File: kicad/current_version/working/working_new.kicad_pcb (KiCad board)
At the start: 2 copper layers, 34 parts, among them J1 bbat328, J2 hi12x3p, J3 scumnsmo, U1 itq32at328, U2 pms22311171d5v, U3 isp16ch340g, X1 xcr3213mhz16, X2 xcr3213mhz12

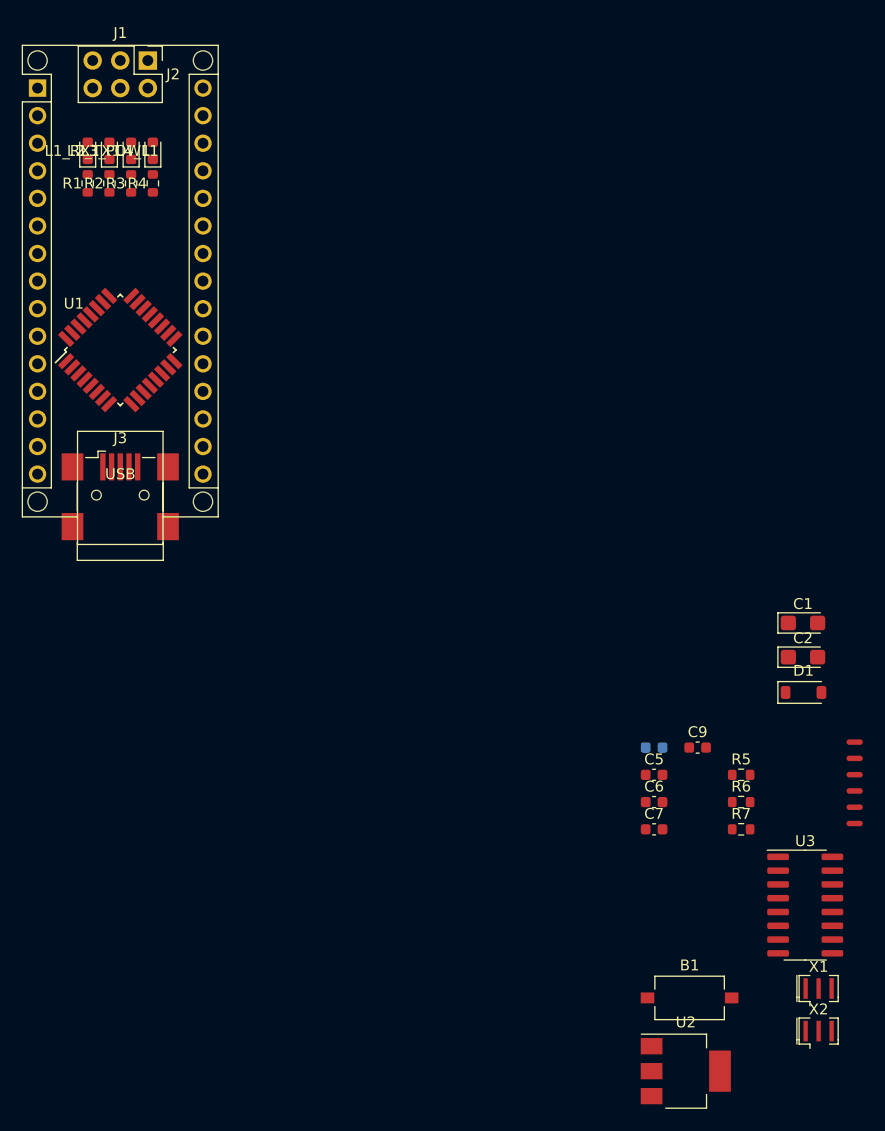
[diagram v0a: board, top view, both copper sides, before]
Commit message: workings
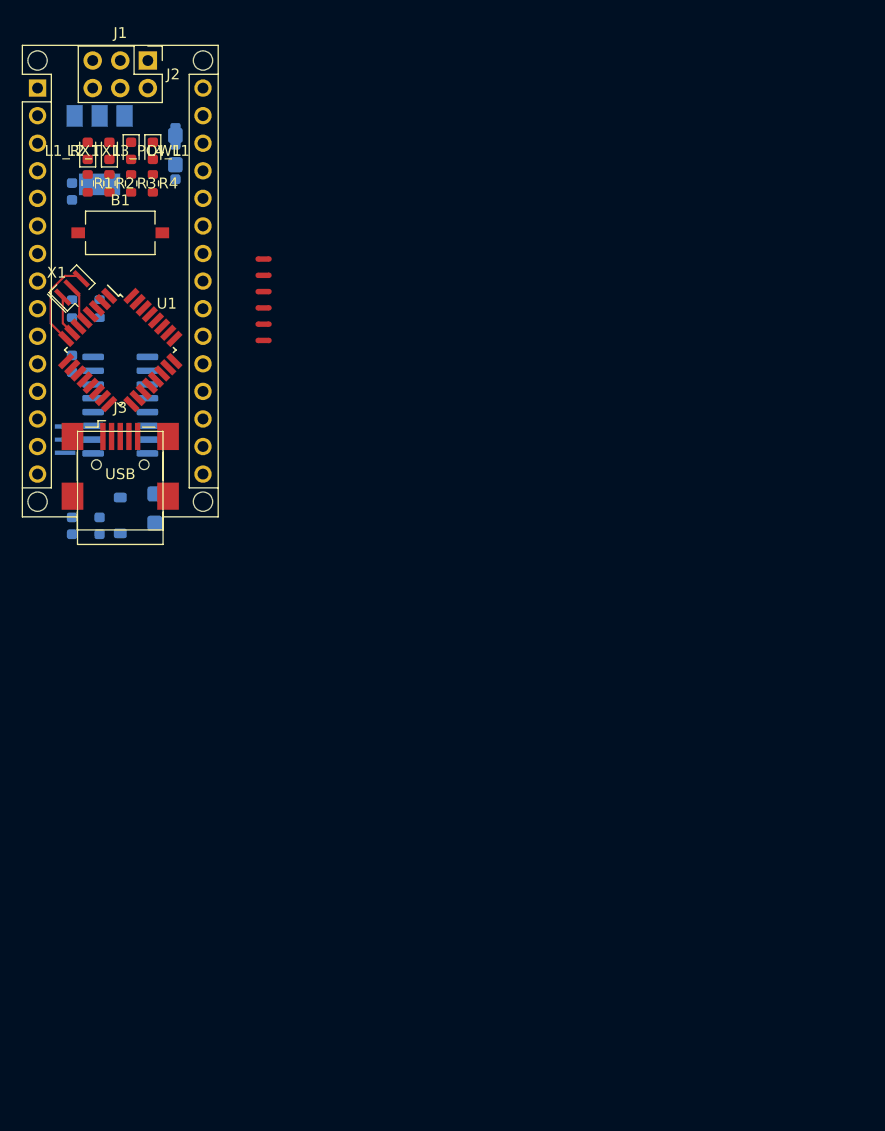
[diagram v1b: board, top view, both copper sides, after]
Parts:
- removed C9: c6nf100, oomlout_oomp_part_footprints:c6nf100_electronic_capacitor_0603_100_nano_farad
- added C4: c6nf100, oomlout_oomp_part_footprints:c6nf100_electronic_capacitor_0603_100_nano_farad, B.Cu at (-4.45, 22.5)
- C1, C2, C5, C6, C7, D1, R5, R6, R7, U2, U3, X2: moved to B.Cu
- moved U2 100.6 mm to (-1.91, -12.1), turned to -90 degrees
- moved X1 94.3 mm to (-4.45, 0.64), turned to 45 degrees
- moved X2 88.2 mm to (-5.08, 14.6), turned to 90 degrees
- moved B1 87.9 mm to (0.00, -4.45)
- moved R7 82.4 mm to (5.08, -13.3), turned to 90 degrees
- moved U3 78.1 mm to (0.00, 11.4)
- moved C6 77.7 mm to (-4.45, -8.26), turned to 90 degrees
- moved R5 75.1 mm to (-4.45, 2.54), turned to 90 degrees
- moved R6 74.6 mm to (-1.91, 2.54), turned to 90 degrees
- moved C2 74.3 mm to (5.08, -12.1), turned to 90 degrees
- moved C5 71.0 mm to (5.08, -10.2), turned to 90 degrees
- moved 1111 70.3 mm to (13.2, -2.03)
- moved 11111 70.3 mm to (13.2, -0.53)
- moved nt1 70.3 mm to (13.2, 0.97)
- moved nt2 70.3 mm to (13.2, 2.47)
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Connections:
- net /pc0 renamed /adc0
- net /pc1 renamed /adc1
- net /pc2 renamed /adc2
- net /pc3 renamed /adc3
- B1 pad 2: +5V -> GND
- C1 pad 2: +5V -> GND
- C2 pad 2: +5V -> GND
- C3 pad 2: +5V -> GND
- C6 pad 2: +5V -> GND
- C7 pad 2: +5V -> GND
- J1 pad 29: +5V -> GND
- J1 pad 4: +5V -> GND
- J2 pad 1: unconnected-(J2-Pin_1-Pad1) -> /miso
- J2 pad 3: unconnected-(J2-Pin_3-Pad3) -> /pb5
- J2 pad 5: unconnected-(J2-Pin_5-Pad5) -> /pc6
- J2 pad 6: +5V -> GND
- J3 pad 5: +5V -> GND
- J3 pad 6: +5V -> GND
- L3_POW1 pad 1: +5V -> GND
- L4_L1 pad 1: +5V -> GND
- U1 pad 21: +5V -> GND
- U1 pad 3: +5V -> GND
- U1 pad 5: +5V -> GND
- U2 pad 1: +5V -> GND
- U3 pad 1: +5V -> GND
- U3 pad 7: /xtal_1 -> /xtal1_ch340
- U3 pad 8: /xtal_2 -> /xtal2_ch340
- X1 pad 1: /xtal_1_atmega328 -> /pb6
- X1 pad 2: +5V -> GND
- X1 pad 3: /xtal_2_atmega328 -> /pb7
- X2 pad 1: /xtal_1_ch340 -> /xtal1_ch340
- X2 pad 2: +5V -> GND
- X2 pad 3: /xtal_2_ch340 -> /xtal2_ch340
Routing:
- net /pb7: track 0.00 -> 8.55 mm
- net /pb6: track 0.00 -> 3.64 mm
- net GND: track 0.00 -> 3.47 mm
